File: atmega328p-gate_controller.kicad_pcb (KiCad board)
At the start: 2 copper layers, 56.4 x 49.1 mm, 24 parts, among them J1 CONN, J10 PWR, J11 Conn_02x04_Counter_Clockwise, J12 UART, J17 JMP, J18 ISP/SPI, J2 JMP, J4 Conn_02x04_Counter_Clockwise, J8 CONN, J9 CONN, U2 AMS1117-3.3, U3 Ra-02, Y1 Crystal

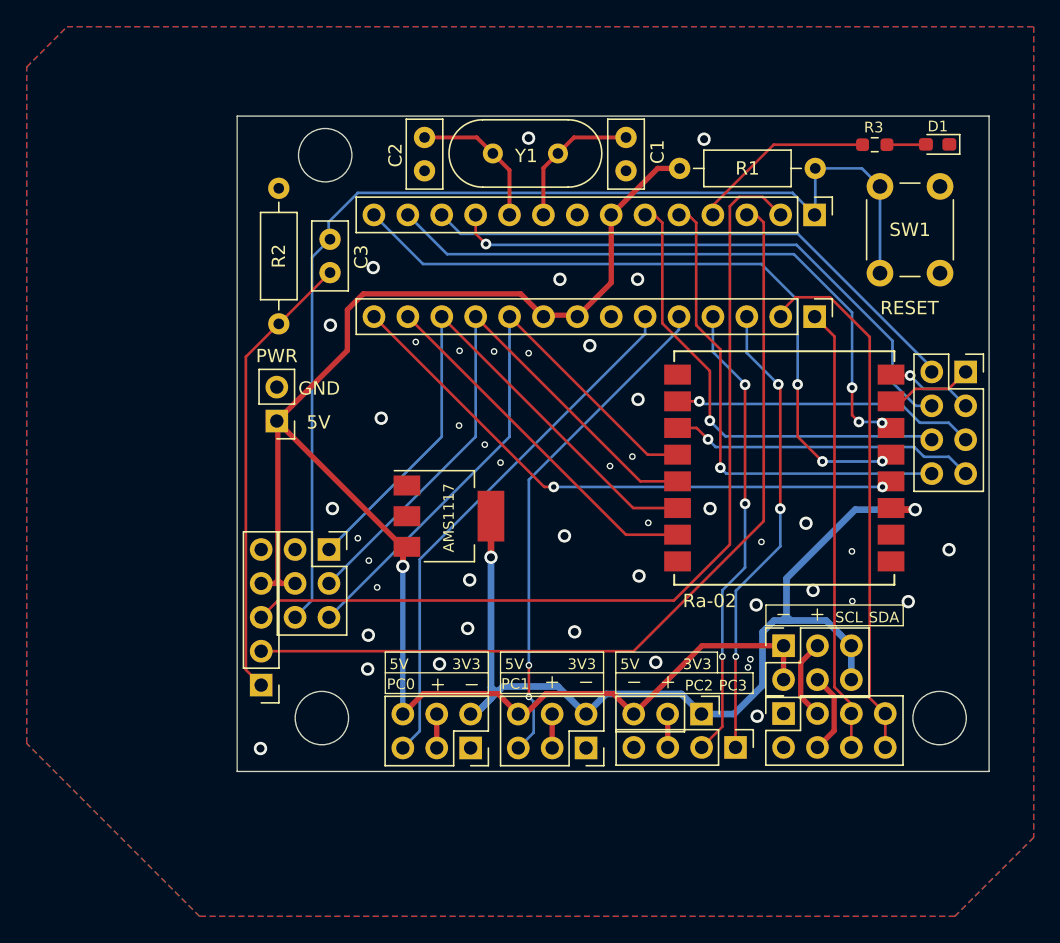
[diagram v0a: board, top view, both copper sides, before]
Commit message: kikit tabs
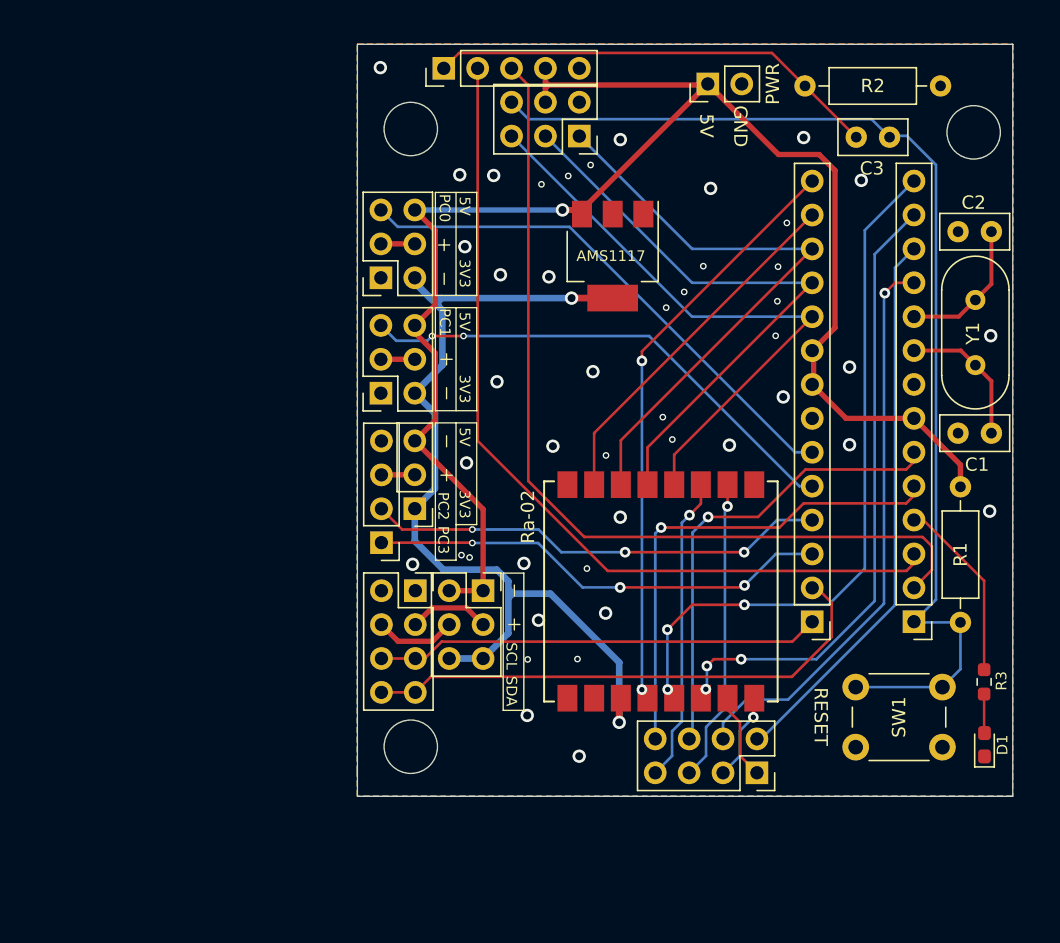
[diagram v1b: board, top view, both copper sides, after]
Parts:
- added REF**: Tab, kikit:Tab, F.Cu at (116.9, 111.6)
- added REF**: Tab, kikit:Tab, F.Cu at (116.9, 54.7)
- added REF**: Tab, kikit:Tab, F.Cu at (144.9, 54.7)
- added REF**: Tab, kikit:Tab, F.Cu at (155.8, 66.1)
- added REF**: Tab, kikit:Tab, F.Cu at (106.0, 100.3)
- added REF**: Tab, kikit:Tab, F.Cu at (144.9, 111.6)
- added REF**: Tab, kikit:Tab, F.Cu at (106.1, 66.1)
- added REF**: Tab, kikit:Tab, F.Cu at (155.8, 100.3)
- moved R2 50.2 mm to (150.0, 58.1), turned to 180 degrees
- moved J12 48.2 mm to (112.8, 56.8), turned to 90 degrees
- moved D1 45.1 mm to (153.3, 107.5), turned to 90 degrees
- moved R3 41.1 mm to (153.3, 102.8), turned to 90 degrees
- moved J10 41.0 mm to (132.6, 58.0), turned to 90 degrees
- moved C3 40.7 mm to (143.7, 62.0), turned to 0 degrees
- moved C2 40.2 mm to (151.4, 69.0), turned to 0 degrees
- moved J18 36.2 mm to (123.0, 61.9), turned to -90 degrees
- moved J8 35.9 mm to (108.1, 72.5), turned to 180 degrees
- moved R1 35.7 mm to (151.5, 98.3), turned to 90 degrees
- moved C1 35.2 mm to (153.9, 84.2), turned to 180 degrees
- moved Y1 35.1 mm to (152.7, 79.0), turned to 90 degrees
- moved J4 33.9 mm to (136.3, 109.6), turned to -90 degrees
- moved REF** 31.4 mm to (148.0, 98.3), turned to 180 degrees
- moved SW1 31.1 mm to (143.7, 103.2), turned to 0 degrees
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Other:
- board size 56.4 x 49.1 mm -> 49.1 x 56.4 mm
